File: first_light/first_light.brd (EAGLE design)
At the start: 160 x 100 mm, 50 parts, among them IC1 MC34063AD, J1 DCJ0202, J2 DCJ0202, Q1 ZXMN4A06GTA, U1 ESP32-WROOM-32D

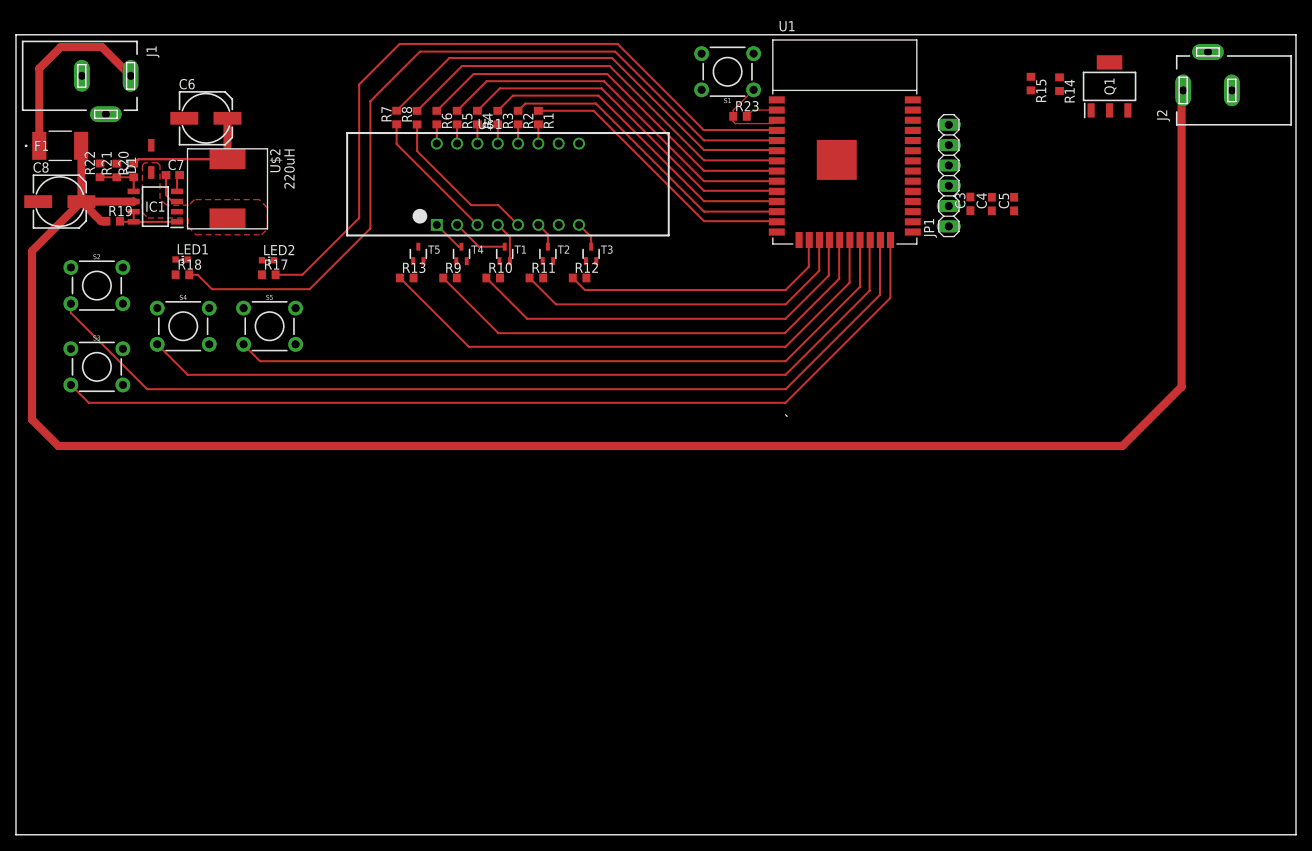
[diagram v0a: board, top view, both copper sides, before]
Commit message: last adjustments before new layout
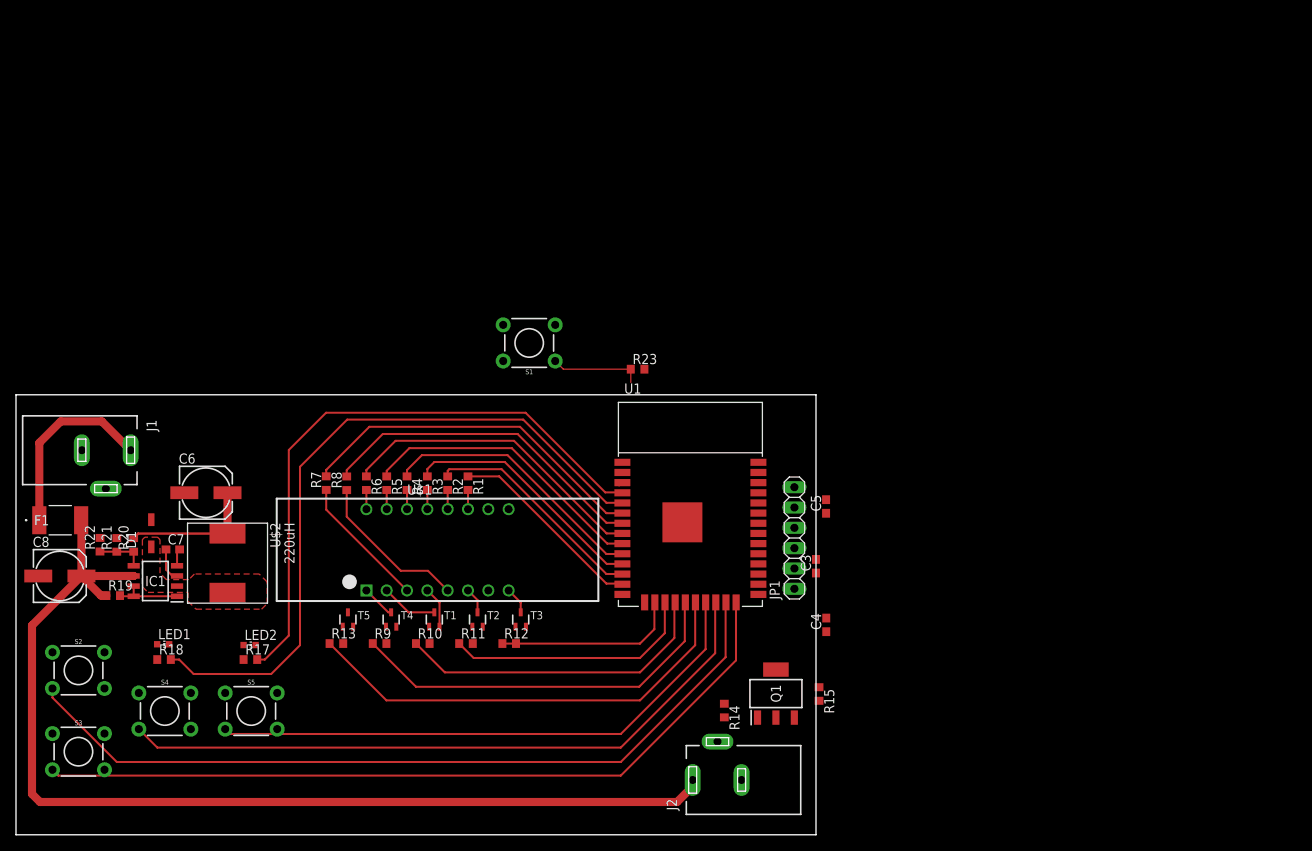
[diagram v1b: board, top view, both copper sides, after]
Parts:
- moved J2 105.8 mm to (87.7, 6.85)
- moved R14 88.8 mm to (88.5, 15.5)
- moved Q1 86.6 mm to (95.0, 17.6)
- moved R15 80.8 mm to (100.4, 17.6)
- moved C4 56.5 mm to (101.3, 26.2)
- moved C3 49.2 mm to (100.0, 33.6)
- moved JP1 49.2 mm to (97.3, 37.1)
- moved U1 49.2 mm to (84.3, 41.3)
- moved LED1 48.2 mm to (18.4, 23.8)
- moved S2 48.2 mm to (7.81, 20.6)
- moved S3 48.2 mm to (7.81, 10.4)
- moved S4 48.2 mm to (18.6, 15.5)
- moved S5 48.2 mm to (29.4, 15.5)
- moved LED2 48.2 mm to (29.2, 23.7)
- moved R17 48.2 mm to (29.3, 21.9)
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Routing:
- net +12V: track 232.7 -> 132.1 mm
- net BTN_UP: track 118.0 -> 100.9 mm
- net BTN_R: track 87.7 -> 70.6 mm
- net BTN_L: track 101.4 -> 84.3 mm
- net BTN_DN: track 116.0 -> 99.0 mm
- net LED_SET: track 88.9 -> 76.2 mm
- net LED_ALM: track 100.4 -> 87.7 mm
- net SSD_D2: track 51.6 -> 40.1 mm
- net SSD_D4: track 34.7 -> 23.1 mm
- net SSD_BLANK: track 68.4 -> 56.9 mm
- net SSD_D3: track 43.2 -> 31.6 mm
- net SSD_D1: track 60.1 -> 48.5 mm
- net SSD_F: track 35.5 -> 24.9 mm
- net SSD_D: track 55.1 -> 44.5 mm
- net SSD_E: track 52.2 -> 41.8 mm
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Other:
- board size 160 x 100 mm -> 100 x 55 mm
